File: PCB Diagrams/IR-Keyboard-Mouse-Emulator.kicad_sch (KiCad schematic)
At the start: 4 parts, among them U1 VS1838B, U2 ProMicroC

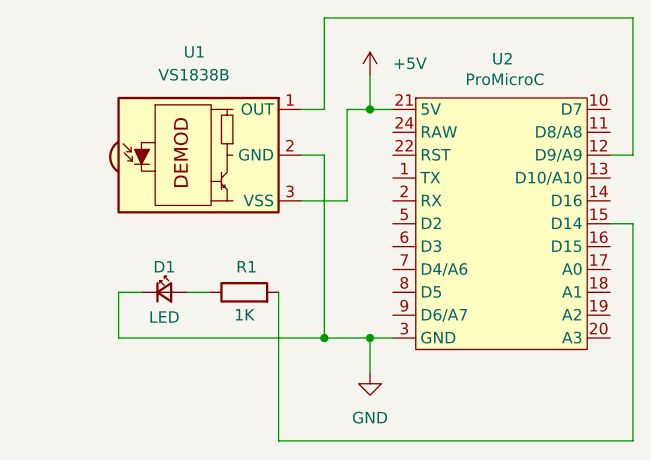
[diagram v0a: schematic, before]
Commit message: update schematics and pcb
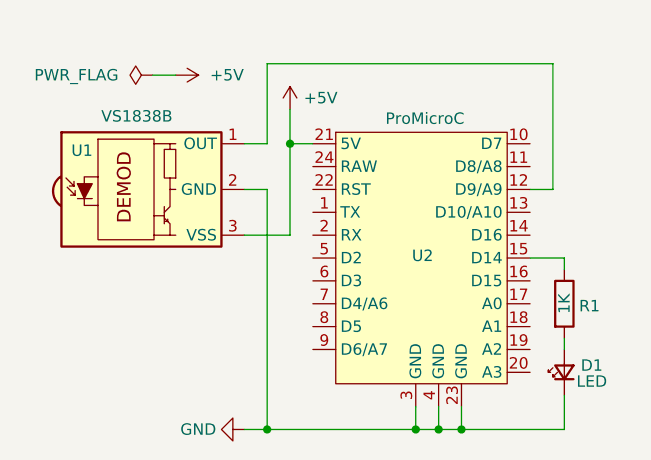
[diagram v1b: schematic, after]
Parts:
- R1: footprint Resistor_THT:R_Axial_DIN0204_L3.6mm_D1.6mm_P5.08mm_Horizontal -> Resistor_THT:R_Axial_DIN0207_L6.3mm_D2.5mm_P7.62mm_Horizontal
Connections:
- net at U2.15 (D14): now also R1.1; no longer R1.2
- net at D1.2 (A): now also R1.2; no longer R1.1
- net GND: no longer names the net of D1.1 (K), U1.2 (GND), U2.23 (GND), U2.3 (GND), U2.4 (GND)
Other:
- moved on the sheet: D1, R1, U1
